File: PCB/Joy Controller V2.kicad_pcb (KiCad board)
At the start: 2 copper layers, 172.6 x 66.8 mm, 67 parts, among them J1 USB_C_Receptacle_USB2.0_16P, J2 Conn_02x16_Odd_Even, Q1 NPN, Q2 NPN, SW1 SW_Push, SW10 SW_Push, SW11 SW_Push, SW12 SW_Push, SW13 SW_Push, SW14 RotaryEncoder_Switch_MP, SW15 SW_Push, SW2 SW_Push, SW3 SW_Push, SW4 SW_Push, SW5 SW_Push, SW6 SW_Push, SW7 SW_Push, SW8 SW_Push, SW9 SW_Push, U1 COM-09032, U2 COM-09032, U3 MCP23017_SO, U4 ADS1015IDGS

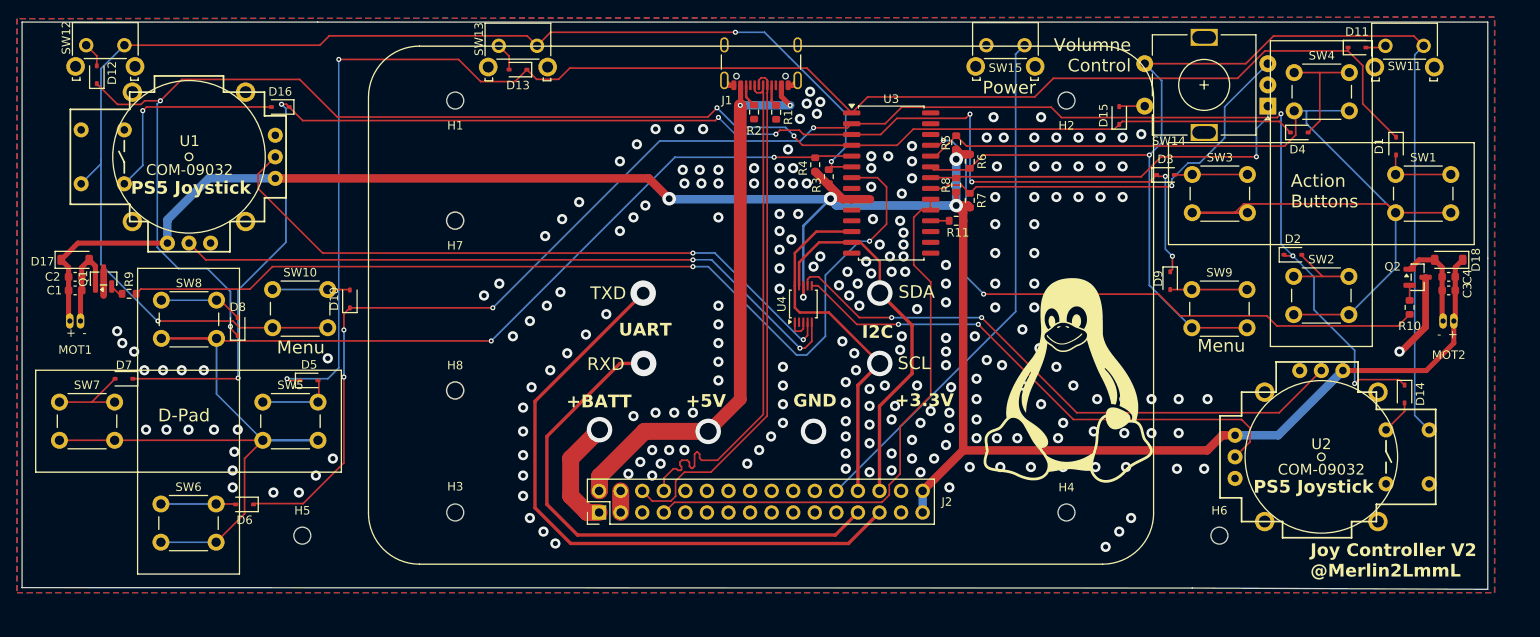
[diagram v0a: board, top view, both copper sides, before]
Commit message: Add files via upload
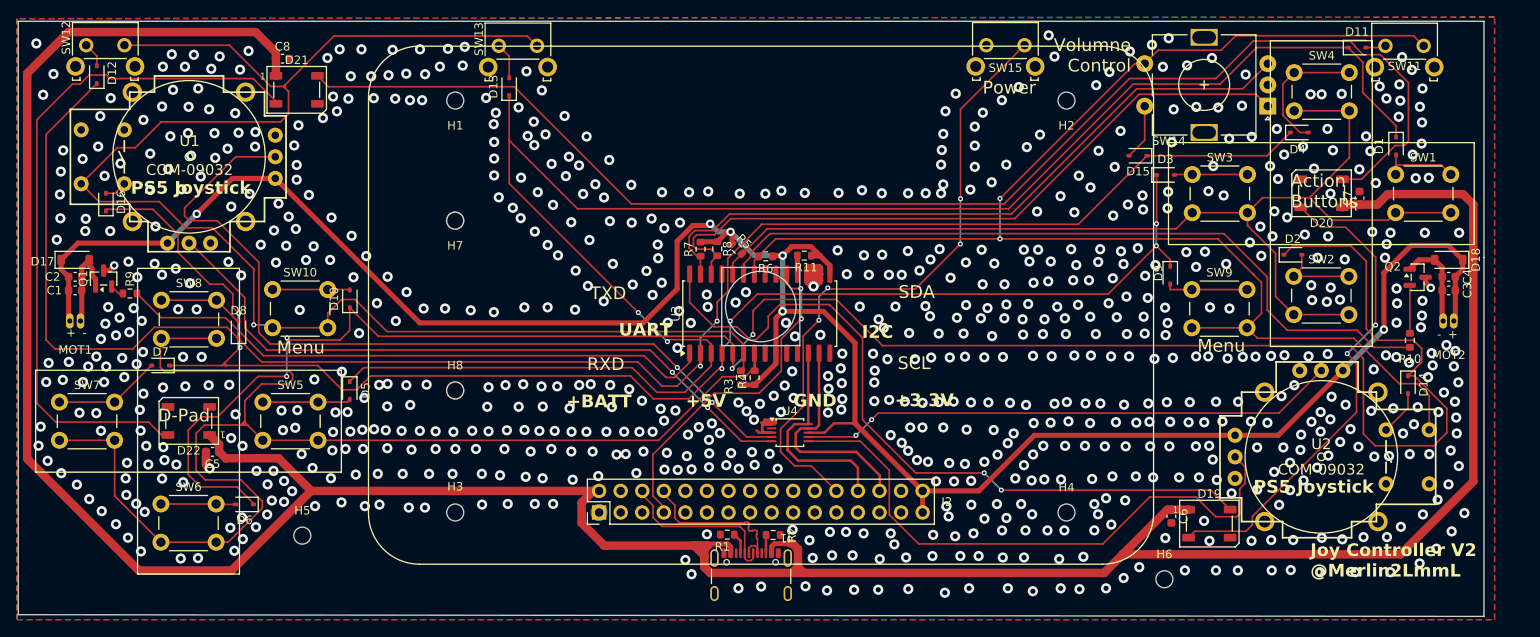
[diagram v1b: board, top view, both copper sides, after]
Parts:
- removed G***: LOGO, Joy:Penguin
- added C5: 100nF, Capacitor_SMD:C_0603_1608Metric, F.Cu at (65.0, 115.6)
- added C6: 100nF, Capacitor_SMD:C_0603_1608Metric, F.Cu at (177.9, 123.2)
- added C7: 100nF, Capacitor_SMD:C_0603_1608Metric, F.Cu at (200.1, 85.7)
- added C8: 100nF, Capacitor_SMD:C_0603_1608Metric, F.Cu at (73.3, 69.3)
- added D19: WS2812B, LED_SMD:LED_WS2812B_PLCC4_5.0x5.0mm_P3.2mm, F.Cu at (182.4, 124.1)
- added D20: WS2812B, LED_SMD:LED_WS2812B_PLCC4_5.0x5.0mm_P3.2mm, F.Cu at (195.6, 85.2)
- added D21: WS2812B, LED_SMD:LED_WS2812B_PLCC4_5.0x5.0mm_P3.2mm, F.Cu at (74.9, 73.0)
- added D22: WS2812B, LED_SMD:LED_WS2812B_PLCC4_5.0x5.0mm_P3.2mm, F.Cu at (62.2, 112.0)
- moved J1 62.5 mm to (128.4, 131.2), turned to 0 degrees
- moved R1 50.1 mm to (125.7, 125.4), turned to 180 degrees
- moved R2 49.9 mm to (131.1, 125.4), turned to 0 degrees
- moved R7 32.2 mm to (122.5, 91.7), turned to -90 degrees
- moved R8 29.1 mm to (124.5, 91.7), turned to -90 degrees
- moved R5 28.7 mm to (126.8, 91.7), turned to -45 degrees
- moved R6 26.5 mm to (130.2, 92.6), turned to 180 degrees
- moved R4 26.1 mm to (128.9, 106.9)
- moved R3 25.8 mm to (127.2, 106.9)
- moved D16 23.4 mm to (52.5, 86.2), turned to 90 degrees
- moved U3 21.8 mm to (129.5, 99.3), turned to 90 degrees
- moved R11 18.3 mm to (134.7, 92.5)
- moved U4 15.2 mm to (133.0, 113.3), turned to 0 degrees
- moved H6 8.27 mm to (177.1, 130.6)
- moved D15 5.23 mm to (174.0, 80.7), turned to 180 degrees
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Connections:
- U3 pad 1: ROW0 -> M_HAP_L
- U3 pad 15: GND -> +3.3V
- U3 pad 2: ROW1 -> ROW3
- U3 pad 21: ROT_ENC_B -> unconnected-(U3-GPA0-Pad21)
- U3 pad 22: ROT_ENC_A -> COL0
- U3 pad 23: COL0 -> M_HAP_R
- U3 pad 25: M_HAP_R -> unconnected-(U3-GPA4-Pad25)
- U3 pad 26: TH1 -> ROT_ENC_A
- U3 pad 27: unconnected-(U3-GPA6-Pad27) -> ROT_ENC_B
- U3 pad 28: unconnected-(U3-GPA7-Pad28) -> LEDs
- U3 pad 3: ROW2 -> ROW0
- U3 pad 4: ROW3 -> ROW2
- U3 pad 5: COL2 -> ROW1
- U3 pad 7: M_HAP_L -> COL2
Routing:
- net +5V: track 70.5 -> 368.3 mm, vias 3 -> 0
- net Net-(D20-DOUT): track 0.00 -> 161.3 mm
- net LEDs: track 0.00 -> 86.9 mm, vias 0 -> 2
- net Net-(D21-DOUT): track 0.00 -> 82.3 mm
- net TXD(GPIO43): track 74.4 -> 0.00 mm, vias 1 -> 0
- net RXD(GPIO44): track 62.2 -> 0.00 mm, vias 1 -> 0
- net Net-(D19-DOUT): track 0.00 -> 57.8 mm, vias 0 -> 2
- net DP: track 61.4 -> 19.2 mm
- net M_HAP_L: track 113.6 -> 71.8 mm, vias 2 -> 0
- net DN: track 62.5 -> 20.8 mm
- net ROW1: track 194.2 -> 235.8 mm, vias 7 -> 4
- net ROT_ENC_A: track 46.0 -> 81.9 mm, vias 1 -> 0
- net ROT_ENC_B: track 50.2 -> 81.8 mm, vias 1 -> 0
- net ROW0: track 184.2 -> 213.3 mm
- net GPIO38: track 66.6 -> 42.0 mm, vias 0 -> 2
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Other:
- board size 172.6 x 66.8 mm -> 172.6 x 70.1 mm
